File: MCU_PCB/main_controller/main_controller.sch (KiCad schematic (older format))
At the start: 47 parts, among them J1 TB006-508-05BE, J2 TB006-508-05BE, J4 TB006-508-05BE, J5 1715250000, SW1 SW_SPDT, U1 STM32F446ZET6, Y1 Crystal_GND24_Small

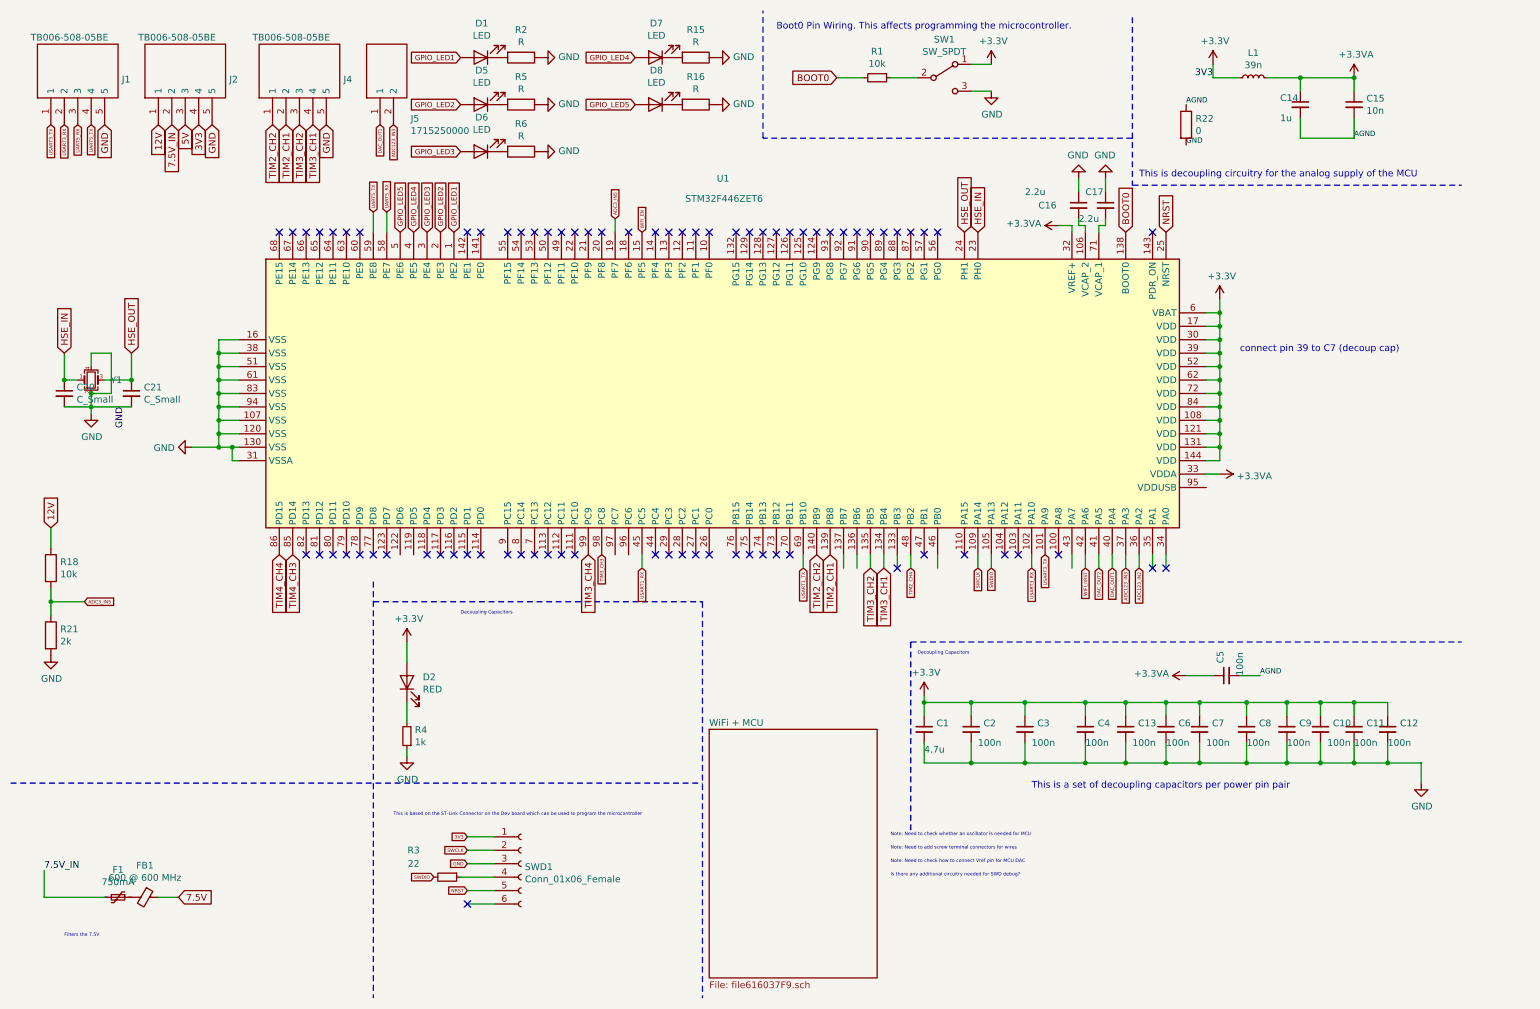
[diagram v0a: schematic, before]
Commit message: Almost approved
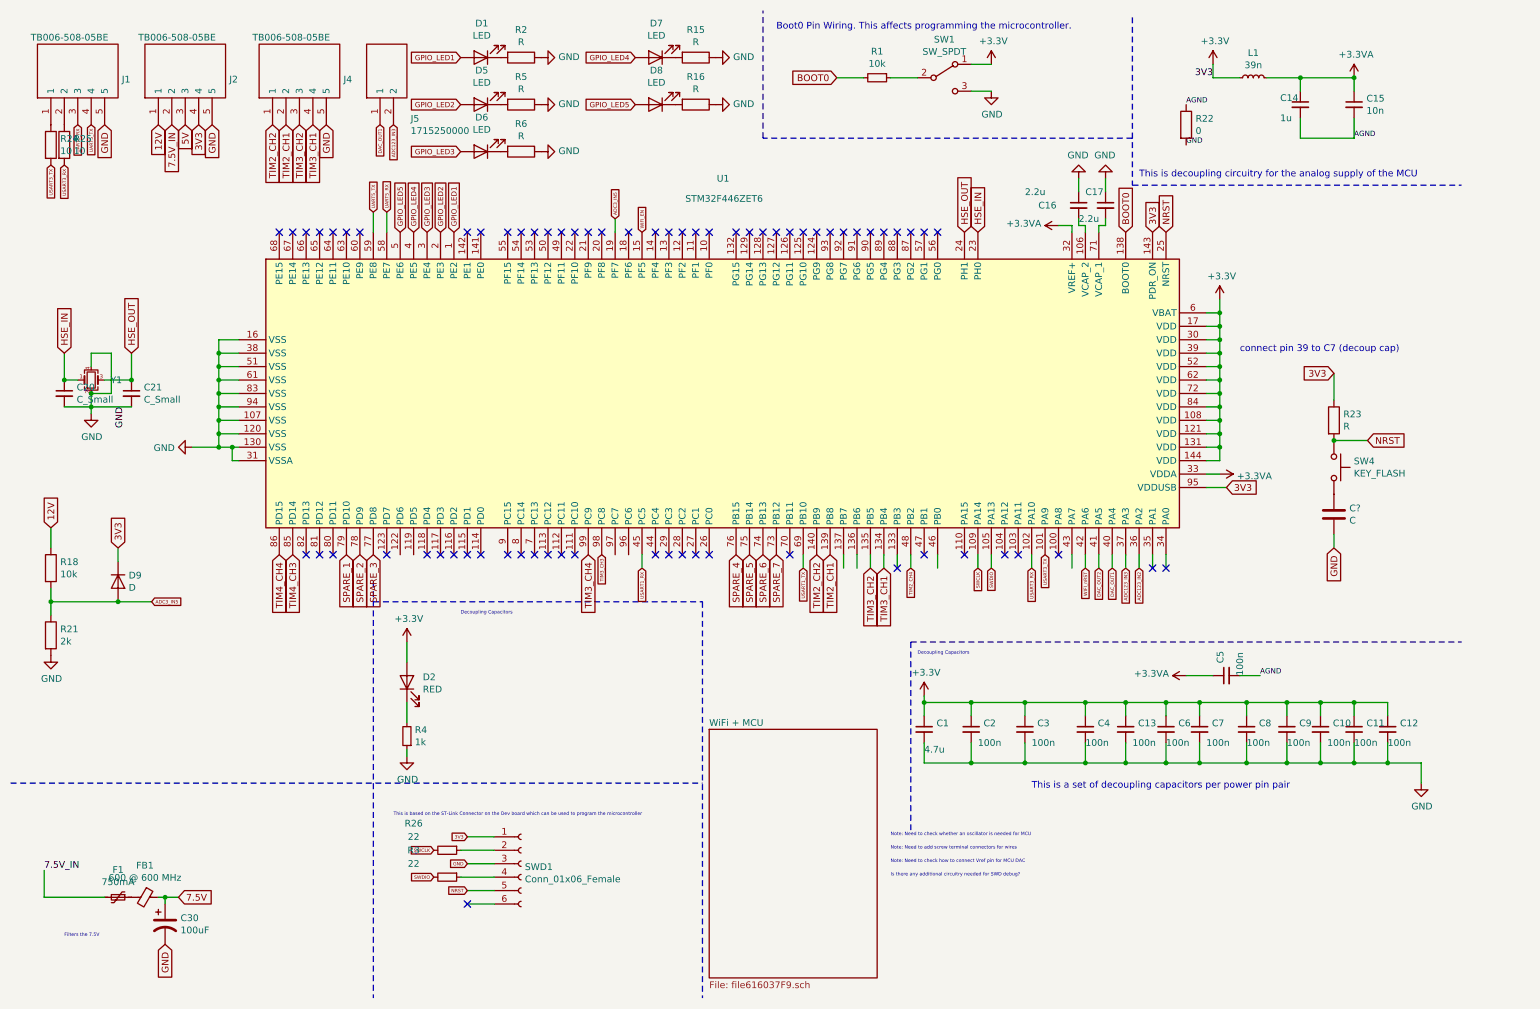
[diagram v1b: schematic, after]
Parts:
- added C30: 100uF, walle_library:CAP_EEEHA0J101WR, symbol Device:CP1
- added C?: C, Capacitor_SMD:C_0805_2012Metric, symbol Device:C
- added D9: D, Diode_SMD:D_0805_2012Metric, symbol Device:D
- added R23: R, Resistor_SMD:R_0805_2012Metric, symbol Device:R
- added R24, R25: 10, Resistor_SMD:R_0805_2012Metric, symbol Device:R
- added R26: 22, Resistor_SMD:R_0805_2012Metric, symbol Device:R_Small
- added SW4: KEY_FLASH, walle_library:SW_147873-2, symbol Switch:SW_Push
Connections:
- net +3V3: now also U1.143 (PDR_ON), U1.95 (VDDUSB), D9.1 (K), R23.1
- net 7.5V: now also C30.1
- net ADC3_IN5: now also D9.2 (A)
- net GND: now also C30.2, C?.2
- net NRST: now also R23.2, SW4.1
- net SWCLK: now also R26.2; no longer SWD1.2 (Pin_2)
- net USART3_RX: now also R25.2; no longer J1.2
- net USART3_TX: now also R24.2; no longer J1.1
- net SPARE_7: now reaches U1.73 (PB12)
- net SPARE_6: now reaches U1.74 (PB13)
- net SPARE_5: now reaches U1.75 (PB14)
- net SPARE_4: now reaches U1.76 (PB15)
- net SPARE_3: now reaches U1.77 (PD8)
- net SPARE_2: now reaches U1.78 (PD9)
- net SPARE_1: now reaches U1.79 (PD10)
- new net: R26.1, SWD1.2 (Pin_2)
- new net: C?.1, SW4.2
- new net: J1.1, R24.1
- new net: J1.2, R25.1
- no-connect marks 77 -> 69
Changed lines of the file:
@@
 	700  7050 1150 7050
 Wire Wire Line
-	1550 7050 1700 7050
+	1550 7050 1600 7050
 Text Notes 850  7350 0    25   ~ 0
 Filters the 7.5V
@@
 	4050 6600 3850 6600
 Wire Wire Line
-	4050 6700 3850 6700
-Wire Wire Line
 	4050 6800 3850 6800
 Wire Wire Line
@@
 Text GLabel 3850 6600 0    25   Input ~ 0
 3V3
-Text GLabel 3850 6700 0    25   Input ~ 0
+Text GLabel 3600 6700 0    25   Input ~ 0
 SWCLK
 Text GLabel 3850 6800 0    25   Input ~ 0
@@
 	0    -1   -1   0
 $EndComp
-Text GLabel 750  1300 3    25   Input ~ 0
+Text GLabel 750  1600 3    25   Input ~ 0
 USART3_TX
-Text GLabel 850  1300 3    25   Input ~ 0
+Text GLabel 850  1600 3    25   Input ~ 0
 USART3_RX
 Text GLabel 950  1300 3    25   Input ~ 0
@@
 NoConn ~ 2750 4500
 NoConn ~ 2850 4500
-NoConn ~ 2950 4500
-NoConn ~ 3050 4500
-NoConn ~ 3150 4500
 NoConn ~ 3250 4500
 NoConn ~ 3550 4500
@@
 NoConn ~ 5350 4500
 NoConn ~ 5250 4500
-NoConn ~ 5850 4500
-NoConn ~ 5950 4500
-NoConn ~ 6050 4500
-NoConn ~ 6150 4500
 NoConn ~ 6250 4500
 NoConn ~ 7550 4500
@@
 NoConn ~ 5950 2100
 NoConn ~ 5850 2100
-NoConn ~ 8950 2100
 Wire Wire Line
 	8350 2100 8350 2050
@@
 Text GLabel 750  4300 1    50   Input ~ 0
 12V
-Wire Wire Line
-	750  4850 1000 4850
 Connection ~ 750  4850
 Wire Wire Line
 	750  4850 750  4950
-Text GLabel 1000 4850 2    25   Input ~ 0
+Text GLabel 1500 4850 2    25   Input ~ 0
 ADC3_IN5
 Text Label 9750 5400 0    39   ~ 0
@@
 GND
 Connection ~ 850  3200
+Wire Wire Line
+	750  4850 1250 4850
+$Comp
+L Device:D D9
+U 1 1 61731FF7
+P 1250 4700
+F 0 "D9" V 1204 4779 50  0000 L CNN
+F 1 "D" V 1295 4779 50  0000 L CNN
+F 2 "Diode_SMD:D_0805_2012Metric" H 1250 4700 50  0001 C CNN
+F 3 "~" H 1250 4700 50  0001 C CNN
+	1    1250 4700
+	0    1    1    0
+$EndComp
+Connection ~ 1250 4850
+Wire Wire Line
+	1250 4850 1500 4850
+Wire Wire Line
+	1250 4550 1250 4450
+Wire Wire Line
+	10300 3150 10300 3350
+Text GLabel 10300 3150 0    50   Input ~ 0
+3V3
+$Comp
+L Device:R R23
+U 1 1 6174F725
+P 10300 3500
+F 0 "R23" H 10370 3546 50  0000 L CNN
+F 1 "R" H 10370 3455 50  0000 L CNN
+F 2 "Resistor_SMD:R_0805_2012Metric" V 10230 3500 50  0001 C CNN
+F 3 "~" H 10300 3500 50  0001 C CNN
+	1    10300 3500
+	1    0    0    -1
+$EndComp
+$Comp
+L Switch:SW_Push SW?
+U 1 1 6175137A
+P 10300 3850
+AR Path="/616037FA/6175137A" Ref="SW?"  Part="1"
+AR Path="/6175137A" Ref="SW4"  Part="1"
+F 0 "SW4" V 10254 3998 50  0000 L CNN
+F 1 "KEY_FLASH" V 10345 3998 50  0000 L CNN
+F 2 "walle_library:SW_147873-2" H 10300 4050 50  0001 C CNN
+F 3 "~" H 10300 4050 50  0001 C CNN
+	1    10300 3850
+	0    1    1    0
+$EndComp
+Wire Wire Line
+	10300 3650 10550 3650
+Connection ~ 10300 3650
+Text GLabel 10550 3650 2    50   Input ~ 0
+NRST
+Wire Wire Line
+	10300 4350 10300 4450
+Text GLabel 10300 4450 3    50   Input ~ 0
+GND
+Text GLabel 1250 4450 1    50   Input ~ 0
+3V3
+Wire Wire Line
+	9350 4000 9500 4000
+Text GLabel 9500 4000 2    50   Input ~ 0
+3V3
+Text GLabel 8950 2100 1    50   Input ~ 0
+3V3
+$Comp
+L Device:CP1 C?
+U 1 1 617A3D21
+P 1600 7250
+AR Path="/616037FA/617A3D21" Ref="C?"  Part="1"
+AR Path="/617A3D21" Ref="C30"  Part="1"
+F 0 "C30" H 1715 7296 50  0000 L CNN
+F 1 "100uF" H 1715 7205 50  0000 L CNN
+F 2 "walle_library:CAP_EEEHA0J101WR" H 1600 7250 50  0001 C CNN
+F 3 "~" H 1600 7250 50  0001 C CNN
+	1    1600 7250
+	1    0    0    -1
+$EndComp
+Text GLabel 1600 7400 3    50   Input ~ 0
+GND
+Wire Wire Line
+	1600 7100 1600 7050
+Connection ~ 1600 7050
+Wire Wire Line
+	1600 7050 1700 7050
+$Comp
+L Device:R_Small R26
+U 1 1 617DDDFC
+P 3700 6700
+F 0 "R26" V 3500 6450 50  0000 C CNN
+F 1 "22" V 3600 6450 50  0000 C CNN
+F 2 "Resistor_SMD:R_0805_2012Metric" H 3700 6700 50  0001 C CNN
+F 3 "~" H 3700 6700 50  0001 C CNN
+	1    3700 6700
+	0    1    1    0
+$EndComp
+Wire Wire Line
+	3800 6700 4050 6700
+$Comp
+L Device:R R24
+U 1 1 61804E56
+P 750 1450
+F 0 "R24" H 820 1496 50  0000 L CNN
+F 1 "10" H 820 1405 50  0000 L CNN
+F 2 "Resistor_SMD:R_0805_2012Metric" V 680 1450 50  0001 C CNN
+F 3 "~" H 750 1450 50  0001 C CNN
+	1    750  1450
+	1    0    0    -1
+$EndComp
+$Comp
+L Device:R R25
+U 1 1 61805DBC
+P 850 1450
+F 0 "R25" H 920 1496 50  0000 L CNN
+F 1 "10" H 920 1405 50  0000 L CNN
+F 2 "Resistor_SMD:R_0805_2012Metric" V 780 1450 50  0001 C CNN
+F 3 "~" H 850 1450 50  0001 C CNN
+	1    850  1450
+	1    0    0    -1
+$EndComp
+Text GLabel 2950 4500 3    50   Input ~ 0
+SPARE_1
+Text GLabel 3050 4500 3    50   Input ~ 0
+SPARE_2
+Text GLabel 3150 4500 3    50   Input ~ 0
+SPARE_3
+Text GLabel 5850 4500 3    50   Input ~ 0
+SPARE_4
+Text GLabel 5950 4500 3    50   Input ~ 0
+SPARE_5
+Text GLabel 6050 4500 3    50   Input ~ 0
+SPARE_6
+Text GLabel 6150 4500 3    50   Input ~ 0
+SPARE_7
+$Comp
+L Device:C C?
+U 1 1 6171B46B
+P 10300 4200
+F 0 "C?" H 10415 4246 50  0000 L CNN
+F 1 "C" H 10415 4155 50  0000 L CNN
+F 2 "Capacitor_SMD:C_0805_2012Metric" H 10338 4050 50  0001 C CNN
+F 3 "~" H 10300 4200 50  0001 C CNN
+	1    10300 4200
+	1    0    0    -1
+$EndComp
 $EndSCHEMATC
